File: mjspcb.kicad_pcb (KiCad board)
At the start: 4 copper layers, 125.7 x 56.5 mm, 148 parts, among them J1 FTDI, J10 Analog, J11 BOOT0, J12 Tag connect, J13 Conn_Coaxial, J14 Lithium Ion, J15 Temp/Hum, J16 BPW34, J17 USB_C_connector, J18 I2C 3V_perm, J19 I2C 5V_SW, J20 Multi, J3 Prototype header, J4 Oled, J5 Conn_01x02_Male, J6 Solar, J7 Particulate matter, J8 Prototype power, J9 Prototype GND, Q1 DMP2035U-7, Q2 DMP2035U-7, SW1 SW_Push, SW2 SW_Push, U1 USBLC-2SC6, U2 LoRa_1262_G-NiceRF, U3 GPS, U4 PrototypeGrid, U5 STM32L072RBTx-meetjestad, U6 MCP73831, Y1 32kHz

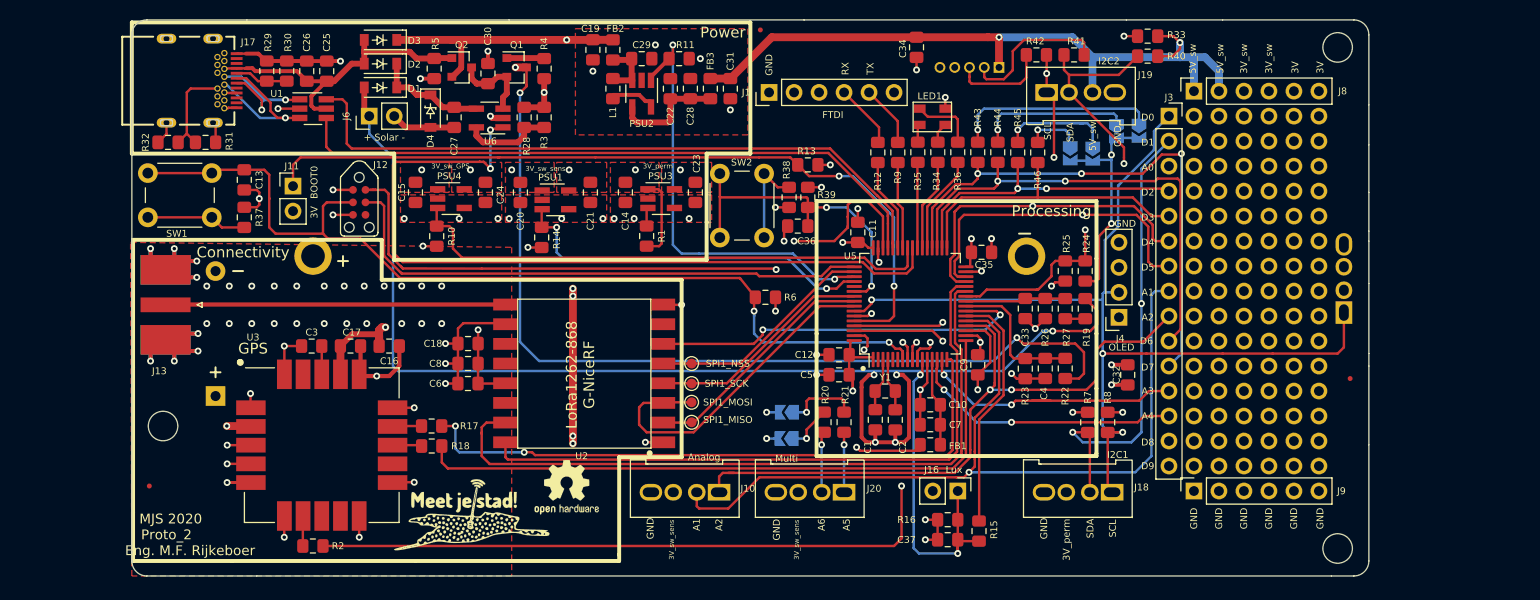
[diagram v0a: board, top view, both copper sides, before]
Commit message: Update to MJS2020-PROTO3
See CHANGELOG.md for detailed changes.
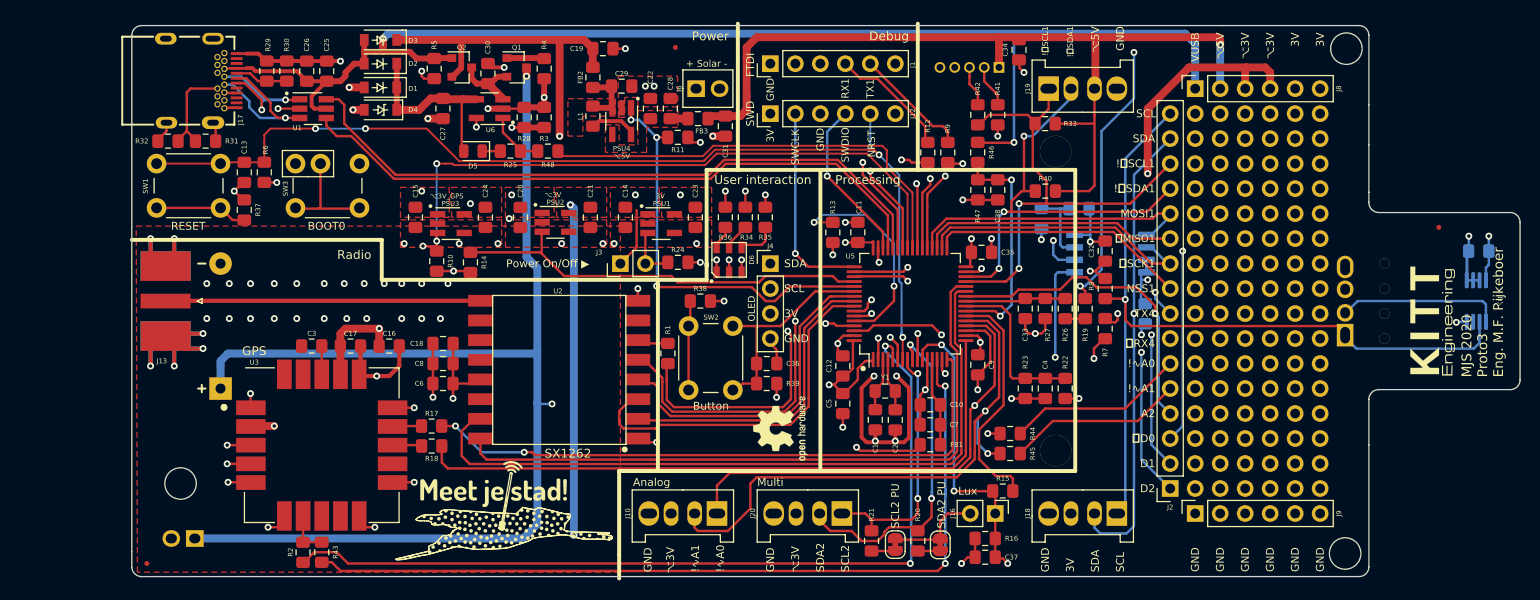
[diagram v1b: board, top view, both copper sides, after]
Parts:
- removed J11: BOOT0, Connector_PinHeader_2.54mm:PinHeader_1x02_P2.54mm_Vertical
- removed LED1: JT-S3030_RGB_LED, meetjestad:JT-S3030_RGB_LED
- removed the PSU1 at (122.9, 79.9)
- removed SP3, SP4, SP5, SP6: SolderJumper_2_Open, Jumper:SolderJumper-2_P1.3mm_Open_TrianglePad1.0x1.5mm
- removed TP1, TP2, TP3, TP4: TestPoint_Small, TestPoint:TestPoint_Pad_D1.0mm
- added C38: 100nF, Capacitor_SMD:C_0805_2012Metric_Pad1.15x1.40mm_HandSolder, F.Cu at (167.9, 78.9)
- added C39: 100nF, Capacitor_SMD:C_0805_2012Metric_Pad1.15x1.40mm_HandSolder, B.Cu at (216.8, 85.1)
- added C40: 100nF, Capacitor_SMD:C_0805_2012Metric_Pad1.15x1.40mm_HandSolder, B.Cu at (182.9, 91.4)
- added D5: LED, LED_SMD:LED_0805_2012Metric, F.Cu at (114.6, 74.9)
- added D6: LED_RGB, meetjestad:JTS3535, F.Cu at (140.6, 86.0)
- added J2: Conn_01x16_Female, Connector_PinSocket_2.54mm:PinSocket_1x16_P2.54mm_Vertical, F.Cu at (185.4, 109.2)
- added Logo_mjs3: Logo_Open_Hardware_Small, meetjestad:mjs-logo-22mm, F.Cu at (106.7, 106.4)
- added Logo_mjs4: Logo_Open_Hardware_Small, Symbol:OSHW-Logo2_7.3x6mm_SilkScreen, B.Cu at (180.8, 75.9)
- added PSU2: TPS7A02, Package_TO_SOT_SMD:SOT-23-5_HandSoldering, F.Cu at (122.9, 82.2)
- added R47: 1M, Resistor_SMD:R_0805_2012Metric_Pad1.15x1.40mm_HandSolder, F.Cu at (165.9, 78.9)
- added R48: 10k, Resistor_SMD:R_0805_2012Metric_Pad1.15x1.40mm_HandSolder, F.Cu at (122.2, 74.9)
- added R49: 10k, Resistor_SMD:R_0805_2012Metric_Pad1.15x1.40mm_HandSolder, B.Cu at (172.3, 81.8)
- added R50: 10k, Resistor_SMD:R_0805_2012Metric_Pad1.15x1.40mm_HandSolder, B.Cu at (176.2, 80.8)
- added SW3: SW_Push, meetjestad:Switch_Header2.54_Combi, F.Cu at (96.5, 76.2)
- added U7: MCP9808_MSOP, Package_SO:MSOP-8_3x3mm_P0.65mm, B.Cu at (216.5, 90.2)
- added U8: SST26VF032B, Package_SO:SOIJ-8_5.3x5.3mm_P1.27mm, B.Cu at (179.4, 85.3)
- H1, H2, H3: footprint meetjestad:Mounting_hole -> MountingHole:MountingHole_3.2mm_M3
- J10, J18, J19, J20: footprint meetjestad:Grove_4pin&Header_4pin -> meetjestad:2,54_2.0pitchCombi
- J12: value Tag connect -> SWD; footprint meetjestad:Tag connect -> Connector_PinHeader_2.54mm:PinHeader_1x06_P2.54mm_Vertical
- J14: footprint meetjestad:BatteryHolder_18650-PC2 -> meetjestad:Combi_2.0_2.45pitch_2PIN
- J15: footprint meetjestad:Grove_4pin&Header_4pin -> meetjestad:SI7021
- J17: footprint 632723300011_Eagle_WR-USB_rev20b:632723100011 -> meetjestad:USB-C_new
- J3: value Prototype header -> Conn_01x02_Male; footprint Connector_PinSocket_2.54mm:PinSocket_1x15_P2.54mm_Vertical -> Connector_PinHeader_2.54mm:PinHeader_1x02_P2.54mm_Vertical
- J4: footprint Connector_PinSocket_2.54mm:PinSocket_1x04_P2.54mm_Vertical -> meetjestad:OLED_1.3
- J6: footprint Connector_PinHeader_2.54mm:PinHeader_1x02_P2.54mm_Vertical -> meetjestad:Combi_2.0_2.45pitch_2PIN
- Logo_kitt1: moved to F.Cu
- Logo_mjs1: footprint meetjestad:mjs_logo -> meetjestad:mjs-logo-16mm; moved to B.Cu
- R15: value 10k -> 3k3
- R24: value 1M -> 100k
- R25: value 100k -> 10k
- R34, R35, R36: value 1k -> 3k3
- R43, R44, R45: value 10k -> 1k
- R46: value 10k -> 1M
- SP2: footprint Jumper:SolderJumper-2_P1.3mm_Open_TrianglePad1.0x1.5mm -> Jumper:SolderJumper-2_P1.3mm_Bridged_RoundedPad1.0x1.5mm; moved to F.Cu
- U5: value STM32L072RBTx-meetjestad -> STM32L072RZTx-meetjestad
- e1: renamed from SP1; footprint Jumper:SolderJumper-2_P1.3mm_Open_TrianglePad1.0x1.5mm -> Jumper:SolderJumper-2_P1.3mm_Bridged_RoundedPad1.0x1.5mm; moved to F.Cu
- moved H2 126.2 mm to (203.3, 64.5)
- moved H1 125.7 mm to (84.8, 108.7)
- moved Logo_kitt1 123.2 mm to (208.3, 92.1), turned to 90 degrees
- moved R43 78.1 mm to (99.2, 115.7)
- moved Logo_mjs1 63.5 mm to (175.8, 94.2), turned to 270 degrees
- moved J3 57.7 mm to (129.5, 86.4), turned to 90 degrees
- moved R25 57.7 mm to (118.4, 74.9), turned to 0 degrees
- moved J14 56.1 mm to (86.4, 114.3), turned to 90 degrees
- moved R6 52.5 mm to (93.3, 77.1), turned to 90 degrees
- moved J12 43.1 mm to (144.8, 71.1), turned to 90 degrees
- moved R24 41.4 mm to (135.4, 86.2), turned to 0 degrees
- moved J4 35.9 mm to (144.8, 86.4), turned to 270 degrees
- moved J6 33.3 mm to (137.2, 68.6)
- moved R45 30.6 mm to (169.2, 105.7), turned to 0 degrees
- moved R44 28.6 mm to (169.2, 103.6), turned to 0 degrees
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- renumbered PSU3 to PSU1, PSU4 to PSU3, PSU2 to PSU4
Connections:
- J12 pad 2: PA13 -> PA14
- J12 pad 3: NRST -> GND
- J12 pad 4: PA14 -> PA13
- J12 pad 5: GND -> NRST
- J3 pad 1: PB6 -> Vin
- J3 pad 2: PB7 -> Net-(J3-Pad2)
- J8 pad 1: 5V-sw -> VBUS
- PSU1 pad 3: Net-(PSU3-Pad3) -> Net-(J3-Pad2)
- PSU4 pad 1: PC10 -> PC12
- R1 pad 1: Net-(PSU3-Pad3) -> Net-(R1-Pad1)
- R1 pad 2: Vin -> PC13
- R11 pad 1: PC10 -> PC12
- R2 pad 1: PC2 -> PH0
- R24 pad 1: 3V-sw_sens -> Net-(J3-Pad2)
- R24 pad 2: PB0 -> GND
- R25 pad 1: PB0 -> Net-(D5-Pad1)
- R25 pad 2: GND -> Net-(R25-Pad2)
- R43 pad 1: PB15 -> PA0
- R43 pad 2: Net-(R43-Pad2) -> Net-(R2-Pad2)
- R44 pad 1: PB14 -> PA4
- R45 pad 1: PB13 -> PA5
- R46 pad 1: PB12 -> VBUS
- R46 pad 2: Net-(R46-Pad2) -> PA7
- U2 pad 5: PA15 -> PC2
- U2 pad 6: PA7 -> Net-(R1-Pad1)
- U5 pad 2: Net-(U5-Pad2) -> PC13
- U5 pad 53: Net-(U5-Pad53) -> PC12
- U6 pad 1: PC9 -> Net-(R25-Pad2)
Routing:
- net VBUS: track 37.7 -> 141.6 mm, vias 0 -> 2
- net PH0: track 0.00 -> 87.8 mm, vias 0 -> 2
- net PA0: track 28.0 -> 86.3 mm
- net PA13: track 69.2 -> 17.1 mm, vias 2 -> 1
- net PC12: track 0.00 -> 42.9 mm, vias 0 -> 3
- net PC2: track 83.8 -> 44.8 mm
- net PC13: track 0.00 -> 35.7 mm, vias 0 -> 2
- net PC9: track 80.6 -> 45.3 mm, vias 2 -> 0
- net PA14: track 55.9 -> 20.8 mm, vias 0 -> 1
- net PB7: track 98.4 -> 133.3 mm
- net PA15: track 23.3 -> 54.8 mm, vias 0 -> 2
- net PH1: track 0.00 -> 30.6 mm, vias 0 -> 2
- net PA5: track 87.6 -> 59.7 mm, vias 1 -> 2
- net PB6: track 100.0 -> 125.8 mm, vias 3 -> 2
- net PB15: track 55.5 -> 30.5 mm, vias 3 -> 0
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- added copper zone on F.Cu, net Net-(C22-Pad1)
- added copper zone on F.Cu, net Net-(C29-Pad1)
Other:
- board size 125.7 x 56.5 mm -> 141.1 x 56 mm
- net class PA11 added: clearance 0.15, trace_width 0.25, via_dia 0.7, via_drill 0.35
- net class PA12 added: clearance 0.15, trace_width 0.25, via_dia 0.7, via_drill 0.35
- net class USBC added: clearance 0.15, trace_width 0.25, via_dia 0.7, via_drill 0.35
- rule trace_min: 0.2 -> 0.15
- rule via_min_size: 0.4 -> 0.35
- board text added: "!∿A0"
- board text added: "!∿A1"
- board text added: "!⎍SCL1"
- board text added: "!⎍SDA1"
- board text added: "Analog input Digital input/output I²C with 3V pullups I²C1 with ⌥5V pullups I²C2 with ⌥3V pullups PWM output DAC, not 5V tolerant Analog input Always on power Switchable power Digital I/O"
- board text added: "Ax Dx SDA, SCL !SDA1, !SCL1 SDA2, SCL2 ⎍ !∿ TX4 3V ⌥3V, ⌥5V All except power"
- board text added: "Button"
- board text added: "Debug"
- board text added: "MJS 2020 Proto3 Eng. M.F. Rijkeboer"
- board text added: "MOSI1"
- board text added: "NRST"
- board text added: "NSS1"
- board text added: "Pin legend"
- board text added: "Power On/Off ▶"
- board text added: "RESET"
- board text added: "RX1"
- board text added: "Radio"
- board text added: "SCL1"
- board text added: "SCL2"
- board text added: "SCL2 PU"
- board text added: "SDA1"
- board text added: "SDA2"
- board text added: "SDA2 PU"
- board text added: "SPS030"
- board text added: "SWCLK"
- board text added: "SWD"
- board text added: "SWDIO"
- board text added: "SX1262"
- board text added: "TX1"
- board text added: "TX4"
- board text added: "User interaction"
- board text added: "VUSB"
- board text added: "⌥3V"
- board text added: "⌥3V_GPS"
- board text added: "⌥5V"
- board text added: "⎍D0"
- board text added: "⎍MISO1"
- board text added: "⎍RX4"
- board text added: "⎍SCK1"
- board text removed: "3V_perm"
- board text removed: "3V_sw"
- board text removed: "3V_sw_GPS"
- board text removed: "3V_sw_sens"
- board text removed: "5V_sw"
- board text removed: "A0"
- board text removed: "A1"
- board text removed: "A3"
- board text removed: "A4"
- board text removed: "A5"
- board text removed: "A6"
- board text removed: "Connectivity"
- board text removed: "D0"
- board text removed: "D3"
- board text removed: "D4"
- board text removed: "D5"
- board text removed: "D6"
- board text removed: "D7"
- board text removed: "D8"
- board text removed: "D9"
- board text removed: "I2C1"
- board text removed: "I2C2"
- board text removed: "I2C2_SCL"
- board text removed: "I2C2_SDA"
- board text removed: "LoRa1262-868 G-NiceRF"
- board text removed: "MJS 2020 Proto_2 Eng. M.F. Rijkeboer"
- board text removed: "Particulate matter"
- board text removed: "RX"
- board text removed: "SPI1_MISO"
- board text removed: "SPI1_MOSI"
- board text removed: "SPI1_NSS"
- board text removed: "SPI1_SCK"
- board text removed: "TX"
